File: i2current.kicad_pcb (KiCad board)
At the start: 2 copper layers, 47 x 60 mm, 111 parts, among them J10 QWIIC, J11 QWIIC, J2 USB_C_Receptacle_USB2.0, J3 CONN_BATT, J4 BIG_OUT, J5 EXT_IFACE, J6 Conn_01x10, J7 Conn_01x05, J8 Conn_01x06, J9 Conn_01x06, Q1 AO3400A, Q4 AO3400A, Q5 AO3400A, Q6 AO3400A, Q8 AO3400A, SW3 B2, SW4 B2, SW6 SW_SPDT, U10 SMTSO3030CTJ, U11 TPS56637RPAR, U2 SMTSO3030CTJ, U3 SMTSO3030CTJ, U4 TPS5430DDA, U5 FUSB302B01MPX, U7 ESP32-C3-WROOM-02, U8 BQ25792RQMR, U9 SMTSO3030CTJ

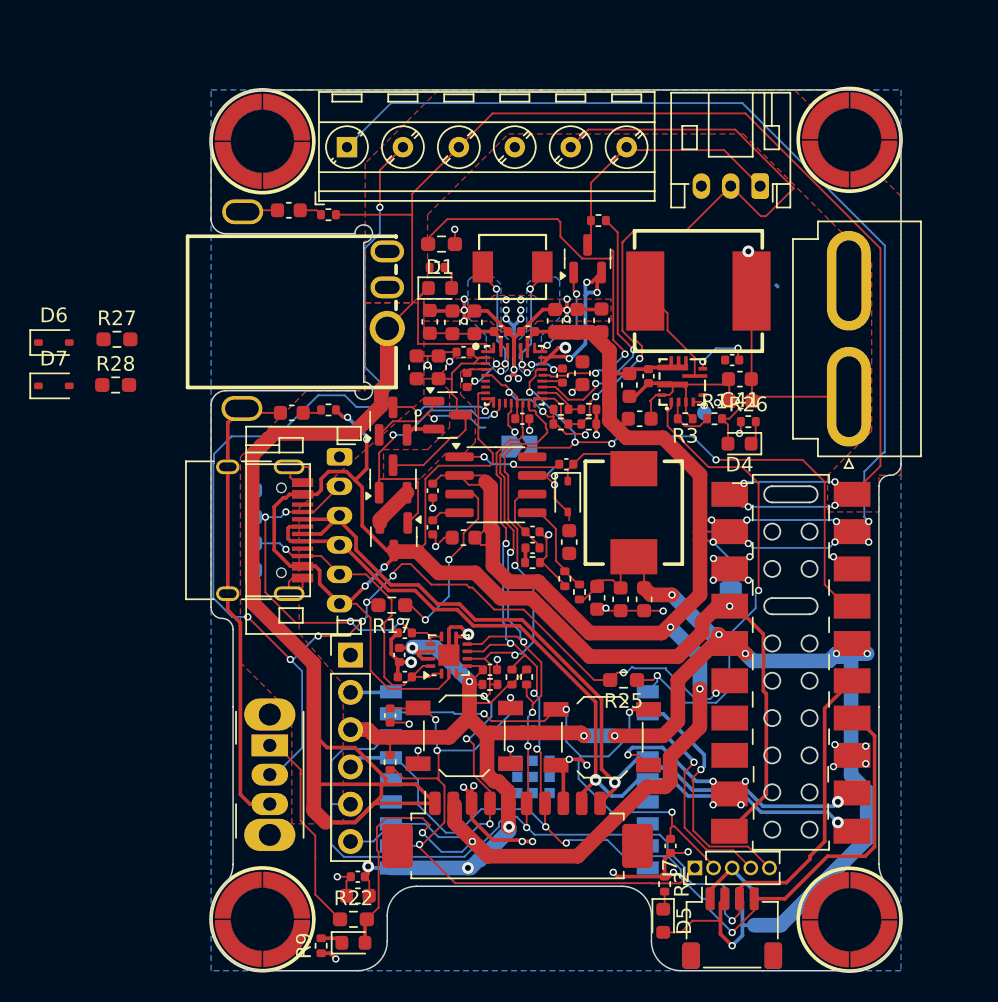
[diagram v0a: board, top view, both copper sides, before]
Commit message: routing 2
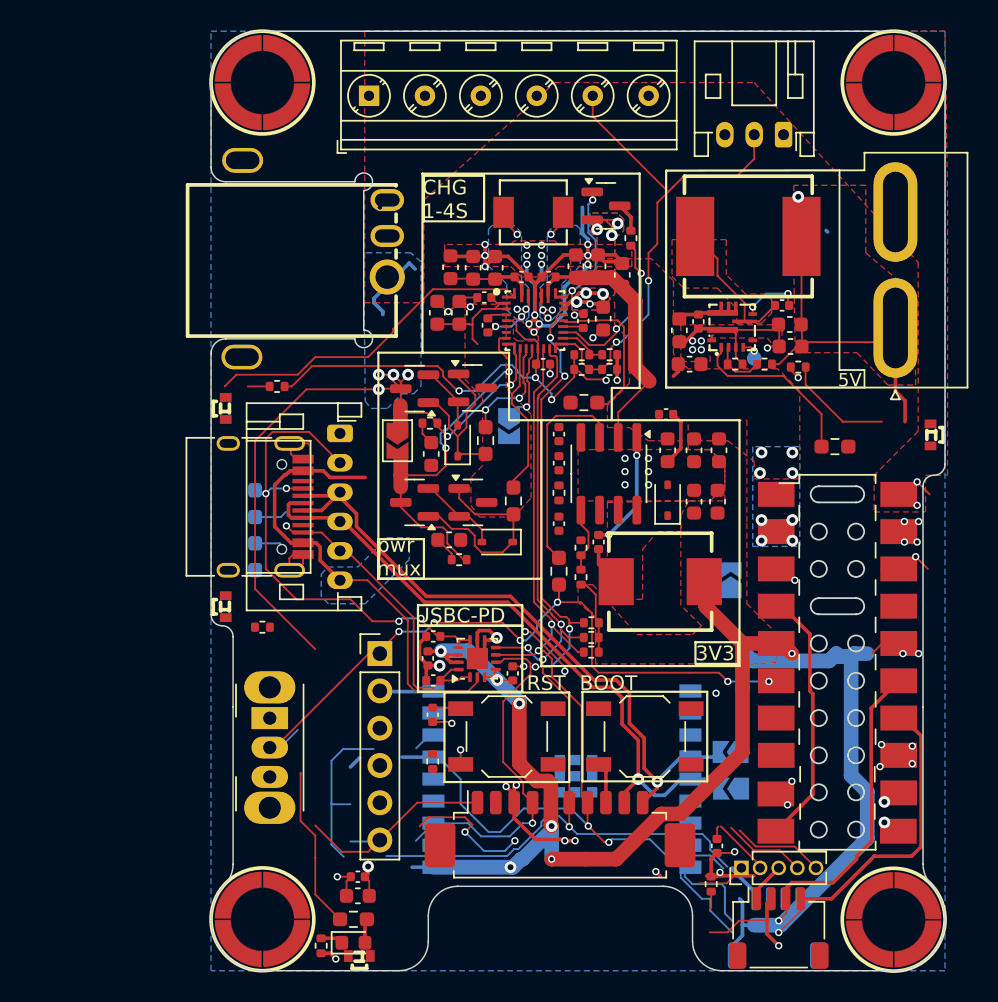
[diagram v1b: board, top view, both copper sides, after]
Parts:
- removed D1, D4, D5: LED, LED_SMD:LED_0603_1608Metric
- added JP3: VBUS_DC, Jumper:SolderJumper-2_P1.3mm_Open_TrianglePad1.0x1.5mm, F.Cu at (60.7, 76.4)
- added JP4: USB_CONN, Jumper:SolderJumper-2_P1.3mm_Open_TrianglePad1.0x1.5mm, B.Cu at (83.4, 100.1)
- added JP5: USB_CONN, Jumper:SolderJumper-2_P1.3mm_Open_TrianglePad1.0x1.5mm, B.Cu at (83.4, 97.6)
- added LED1: XL-1606UGC, easyeda2kicad:LED-SMD_L1.7-W1.1-R-RD_GREEN, F.Cu at (97.0, 76.0)
- added LED2: XL-1606UGC, easyeda2kicad:LED-SMD_L1.7-W1.1-R-RD_GREEN, F.Cu at (58.1, 111.5)
- added LED3: XL-1606UGC, easyeda2kicad:LED-SMD_L1.7-W1.1-R-RD_GREEN, F.Cu at (49.0, 74.2)
- added LED4: XL-1606UGC, easyeda2kicad:LED-SMD_L1.7-W1.1-R-RD_GREEN, F.Cu at (49.0, 87.7)
- added R29: 2k, Resistor_SMD:R_0402_1005Metric, F.Cu at (51.5, 89.1)
- moved D6 33.1 mm to (67.5, 83.3), turned to 180 degrees
- moved R27 29.2 mm to (68.6, 80.5), turned to -90 degrees
- moved D7 27.8 mm to (64.8, 76.4), turned to 90 degrees
- moved R28 25.5 mm to (66.7, 76.4), turned to -90 degrees
- moved R25 21.5 mm to (90.5, 76.8), turned to 0 degrees
- moved C29 19.2 mm to (63.0, 77.3), turned to -90 degrees
- moved C7 16.7 mm to (79.0, 74.6), turned to 180 degrees
- moved R23 15.8 mm to (62.9, 75.2)
- moved C5 15.1 mm to (79.1, 77.0), turned to -90 degrees
- moved R19 14.5 mm to (73.4, 73.8), turned to 0 degrees
- moved C30 13.8 mm to (64.2, 83.2), turned to 0 degrees
- moved R18 13.6 mm to (52.5, 72.7), turned to 180 degrees
- moved R24 13.5 mm to (64.9, 84.5)
- moved C3 13.0 mm to (82.6, 77.0)
- moved R17 11.6 mm to (71.7, 85.3), turned to -90 degrees
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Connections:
- net Net-(D3-K) renamed /3V3_L
- net Net-(U11-SW) renamed /5V_L
- DC1 pad 3: unconnected-(DC1-Pad3) -> GND
- J5 pad 18: /USBIN_M -> Net-(J5-Pin_18)
- J5 pad 20: /USBIN_P -> Net-(J5-Pin_20)
- J8 pad 1: /GLOB_RST -> /GLOB_~{OFF}
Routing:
- net +BATT: track 201.3 -> 41.1 mm, vias 12 -> 14
- net +VDC: track 174.8 -> 66.6 mm, vias 6 -> 8
- net GND: track 185.9 -> 130.6 mm, vias 61 -> 58
- net /GLOB_~{OFF}: track 97.6 -> 47.3 mm, vias 9 -> 6
- net /esp32-c3/ESP_EN: track 47.1 -> 5.54 mm, vias 4 -> 0
- net VBUS: track 109.5 -> 74.0 mm, vias 5 -> 2
- net /esp32-c3/IO9: track 37.2 -> 4.82 mm, vias 4 -> 0
- net /I2C_INT: track 83.6 -> 55.8 mm, vias 9 -> 5
- net /BQ_REGN: track 11.4 -> 33.2 mm, vias 3 -> 4
- net /5V_ENA: track 33.4 -> 12.0 mm, vias 2 -> 1
- net (no net): track 19.9 -> 0.00 mm, vias 2 -> 0
- net Net-(U8-PROG): track 29.1 -> 10.5 mm, vias 2 -> 0
- net /LIPO_NTC: track 51.8 -> 35.7 mm
- net /BAT_IN: track 17.9 -> 2.01 mm
- net /SDA: track 106.3 -> 90.4 mm, vias 6 -> 5
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- added copper zone on F.Cu, net +3.3V
- added copper zone on F.Cu, net +5V
- added copper zone on B.Cu, net +BATT
- added copper zone on F.Cu, net +BATT
- added copper zone on B.Cu, net +VDC
- added copper zone on F.Cu, net /3V3_L
- added copper zone on F.Cu, net /5V_L
- added copper zone on F.Cu, net /BQ_REGN
- added copper zone on B.Cu, net BAT
- added copper zone on F.Cu, net BAT
- added copper zone on B.Cu, net VBUS
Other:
- board size 47 x 60 mm -> 50 x 64 mm
- board text added: "3V3"
- board text added: "5V"
- board text added: "BOOT"
- board text added: "CHG 1-4S"
- board text added: "RST"
- board text added: "USBC-PD"
- board text added: "pwr mux"
